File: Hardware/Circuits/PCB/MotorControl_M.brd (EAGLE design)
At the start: 74.8 x 147 mm, 94 parts, among them IC1 74AHC1G125FDBV, P1 M-2X10-87759, U1 MIC2005, U3 74HC4051BQ, U4 74HC4051BQ

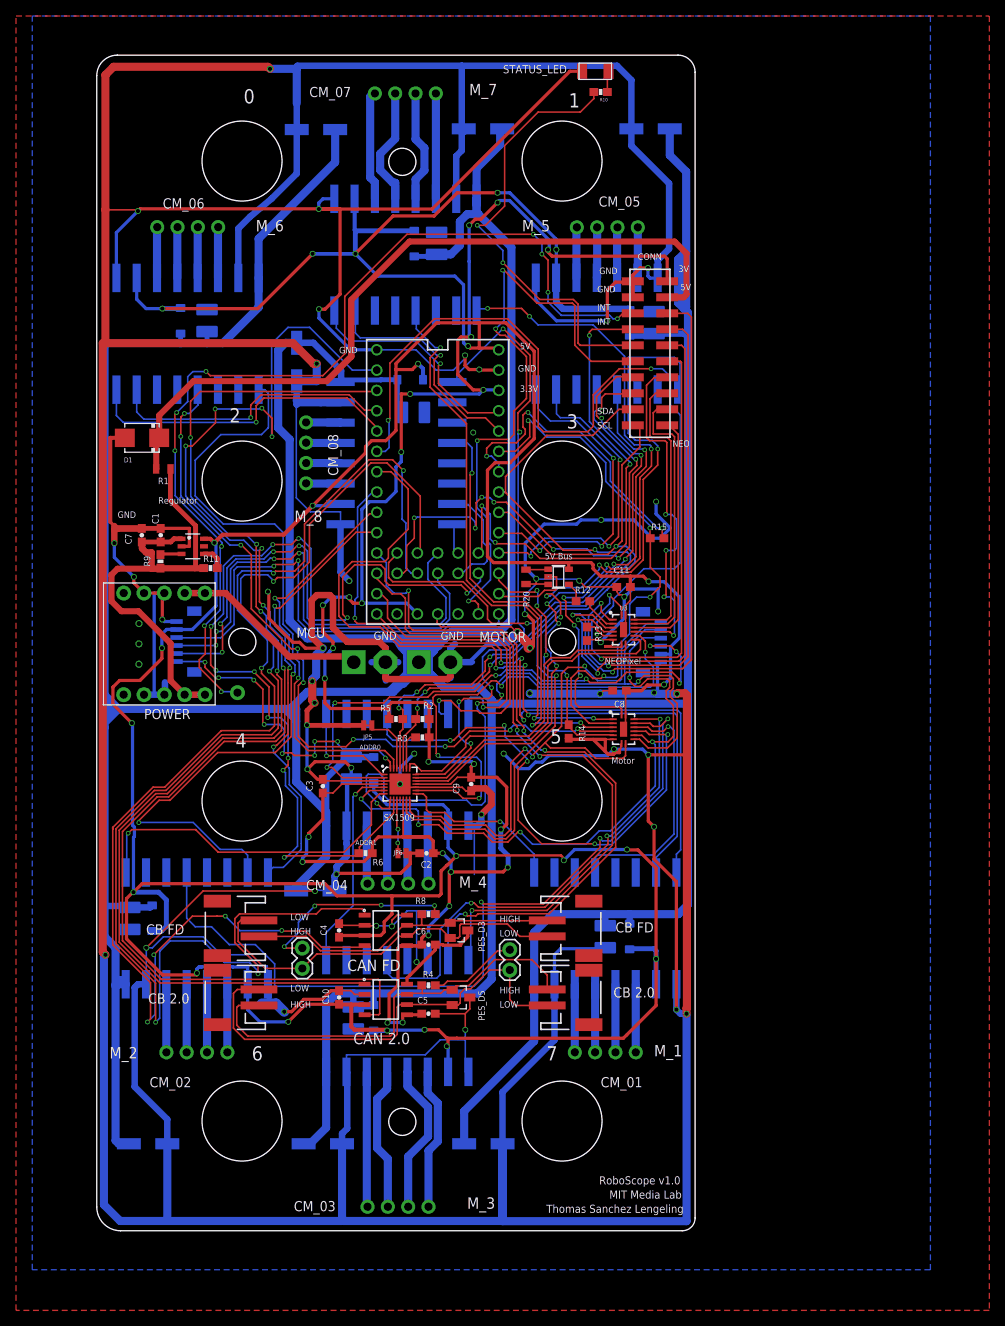
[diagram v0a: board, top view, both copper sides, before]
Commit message: update motors
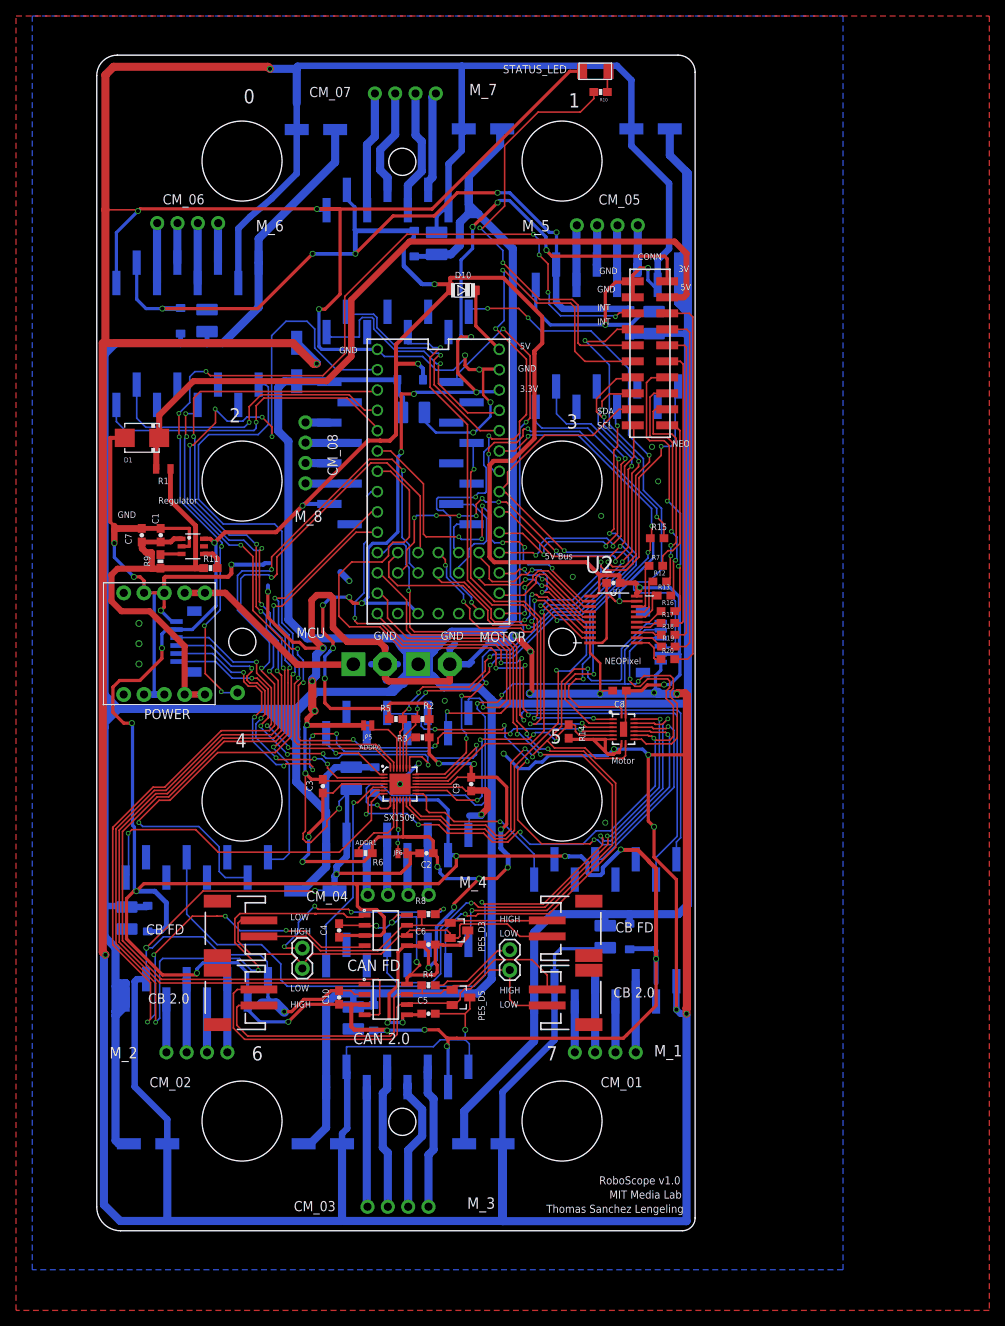
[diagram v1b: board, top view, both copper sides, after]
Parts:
- removed IC1: 74AHC1G125FDBV, 74xx-little-us:SOT23-5
- removed U3: 74HC4051BQ, 8mux:DHVQFN-16-2.5X3.5MM
- added D10: SOD123L, we-rcl:SOD123
- added R16, R17, R18, R19, R7: 100, SparkFun-Resistors:0603
- added U2: 74HCT245D,65220-TSSOP, 74HCT245D_652:20-TSSOP
- C11: value 0.1uF -> 1uf; device SparkFun-Capacitors:0603 -> SparkFun-Capacitors:0603-CAP
- C12: value (none) -> 10uf
- MOTOR_01, MOTOR_02, MOTOR_03, MOTOR_04, MOTOR_05, MOTOR_06, MOTOR_07, MOTOR_08: value DRV8880 -> DRV8880TMC2209; device STSPIN220:DRV8880 -> STSPIN220:TMC2209_SMD
- R13: value 10K -> 100
- R20: value 10K -> 100; device SparkFun-Resistors:0805 -> SparkFun-Resistors:0603
- moved DRILEGEND 89.1 mm to (-89.1, 100.4)
- moved R20 20.5 mm to (71.3, 76.8), turned to 0 degrees
- moved R13 10.7 mm to (70.8, 84.8), turned to 0 degrees
- moved R12 9.91 mm to (70.3, 86.5)
- moved MOTOR_04 1.78 mm to (37.5, 61.2)
- moved CM_04 1.40 mm to (37.6, 47.4)
- moved C11 1.37 mm to (64.5, 86.4)
- moved D5 1.28 mm to (34.7, 61.7)
- moved C19 1.27 mm to (31.8, 62.0)
- moved MOTOR_07 1.25 mm to (37.6, 126.6)
- moved D2 0.56 mm to (6.30, 44.4)
- moved CM_06 0.51 mm to (11.3, 131.3)
- moved MOTOR_08 0.51 mm to (37.9, 102.6)
- moved C12 0.38 mm to (3.68, 44.5)
- moved POWER_M 0.27 mm to (42.1, 76.2)
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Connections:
- removed net INT_03: P1.14, U$3.25
- removed net LIMIT_01: J1.3, U$3.13
- removed net LIMIT_02: J1.4, U$3.28
- removed net LIMIT_03: J1.5, U$3.29
- removed net MOTOR_MUX_E: R14.1, U$3.15/A1, U4.6
- removed net N$4: R12.2, U3.3
- removed net NEO_5V_Z: IC1.4, R12.1
- removed net NEO_MUX_E: R13.1, U$3.4, U3.6
- removed net NEO_TX3: IC1.2, U$3.14/A0
- new net INPUT_02: J4.3, P1.14
- new net N$11: R16.1, U2.15
- new net N$14: R18.1, U2.13
- new net N$15: R19.1, U2.12
- new net N$16: R20.1, U2.11
- new net N$5: D10.C, U$3.VIN
- new net N$6: R7.1, U2.18
- new net N$8: R12.1, U2.17
- new net N$9: R13.1, U2.16
- new net NEOPIXEL_01_3V: U$3.4, U2.2
- new net NEOPIXEL_02_3V: U$3.13, U2.3
- new net NEOPIXEL_03_3V: U$3.14/A0, U2.4
- new net NEOPIXEL_04_3V: U$3.15/A1, U2.5
- new net NEOPIXEL_05_3V: U$3.24, U2.6
- new net NEOPIXEL_06_3V: U$3.25, U2.7
- new net NEOPIXEL_07_3V: U$3.28, U2.8
- new net NEOPIXEL_08_3V: U$3.29, U2.9
- net GND_MCU: now also U2.10, U2.19; no longer IC1.3, R13.2, R20.2, U3.7, U3.8
- net INT_00: no longer U$3.24
- net MOTOR_TX_RX_01: now also MOTOR_01.TX/RX; no longer MOTOR_01.1
- net MOTOR_TX_RX_02: now also MOTOR_02.TX/RX; no longer MOTOR_02.1
- net MOTOR_TX_RX_03: now also MOTOR_03.TX/RX; no longer MOTOR_03.1
- net MOTOR_TX_RX_04: now also MOTOR_04.TX/RX; no longer MOTOR_04.1
- net MOTOR_TX_RX_05: now also MOTOR_05.TX/RX; no longer MOTOR_05.1
- net MOTOR_TX_RX_06: now also MOTOR_06.TX/RX; no longer MOTOR_06.1
- net MOTOR_TX_RX_07: now also MOTOR_07.TX/RX; no longer MOTOR_07.1
- net MOTOR_TX_RX_08: now also MOTOR_08.TX/RX; no longer MOTOR_08.1
- net N$12: now also R17.1, U2.14; no longer IC1.1, R20.1
- net NEOPIXEL_01_5V: now also R7.2; no longer U3.13
- net NEOPIXEL_02_5V: now also R12.2; no longer U3.14
- net NEOPIXEL_03_5V: now also R13.2; no longer U3.15
- net NEOPIXEL_04_5V: now also R16.2; no longer U3.12
- net NEOPIXEL_05_5V: now also R17.2; no longer U3.1
- net NEOPIXEL_06_5V: now also R18.2; no longer U3.5
- net NEOPIXEL_07_5V: now also R19.2; no longer U3.2
- net NEOPIXEL_08_5V: now also R20.2; no longer U3.4
- net SX00_1: now also J1.3; no longer J1.6
- net SX00_11: now also R14.1, U4.6; no longer U3.11
- net SX00_13: now also J1.5; no longer U3.10
- net SX00_15: now also J1.6; no longer U3.9
- net SX00_3: now also J1.4; no longer J4.3
- net VCC_5VREG: now also D10.A, MOTOR_01.5V, MOTOR_02.5V, MOTOR_03.5V, MOTOR_04.5V, MOTOR_05.5V, MOTOR_06.5V, MOTOR_07.5V, MOTOR_08.5V, U2.1, U2.20; no longer IC1.5, MOTOR_01.FAULT, MOTOR_02.FAULT, MOTOR_03.FAULT, MOTOR_04.FAULT, MOTOR_05.FAULT, MOTOR_06.FAULT, MOTOR_07.FAULT, MOTOR_08.FAULT, U$3.VIN, U3.16, U3.EP
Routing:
- net NEO_MUX_E: track 110.8 -> 0.00 mm, vias 3 -> 0
- net INT_00: track 118.5 -> 10.0 mm, vias 11 -> 0
- net LIMIT_03: track 64.2 -> 0.00 mm, vias 4 -> 0
- net INT_03: track 63.8 -> 0.00 mm, vias 4 -> 0
- net LIMIT_02: track 59.6 -> 0.00 mm, vias 4 -> 0
- net LIMIT_01: track 57.8 -> 0.00 mm, vias 2 -> 0
- net INPUT_02: track 0.00 -> 57.2 mm, vias 0 -> 1
- net VCC_5VREG: track 580.5 -> 633.6 mm
- net NEOPIXEL_01_3V: track 0.00 -> 47.1 mm, vias 0 -> 6
- net GND_MCU: track 1347.1 -> 1300.7 mm, vias 53 -> 54
- net VCC_M: track 768.0 -> 804.4 mm
- net SX00_3: track 72.3 -> 39.9 mm, vias 7 -> 5
- net MOTOR_MUX_E: track 32.3 -> 0.00 mm, vias 4 -> 0
- net NEOPIXEL_08_3V: track 0.00 -> 31.5 mm, vias 0 -> 4
- net SX00_11: track 63.7 -> 35.7 mm
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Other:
- board text removed: "01-16"
- board text removed: "LAYER-STACK"
